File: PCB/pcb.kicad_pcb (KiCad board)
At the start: 2 copper layers, 40.2 x 62.5 mm, 7 parts, among them SW1 SW_Push, SW2 SW_Push, SW3 SW_Push, SW4 SW_Push, U1 XIAO-RP2040-DIP

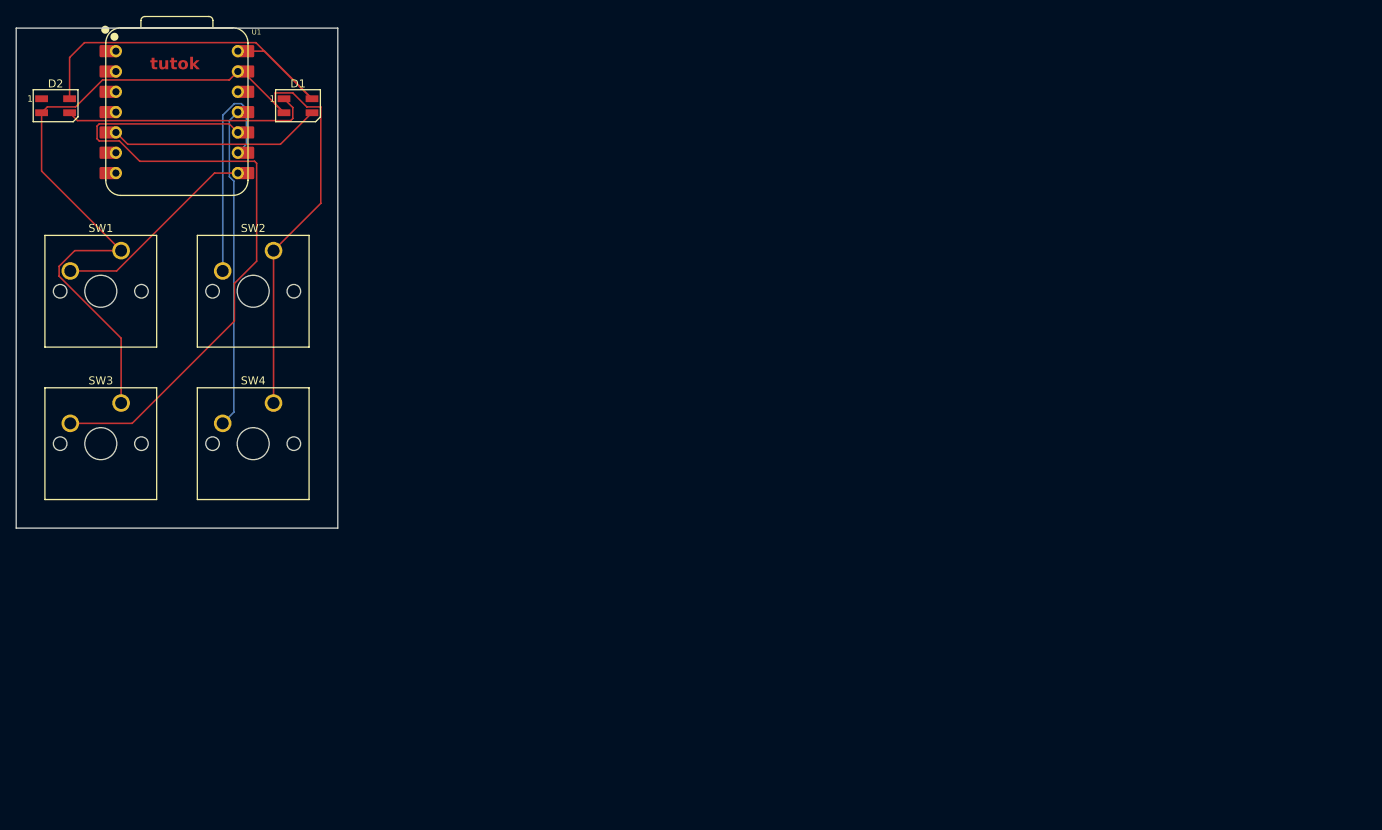
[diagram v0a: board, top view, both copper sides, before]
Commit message: Dodanie nowych plików i zmian
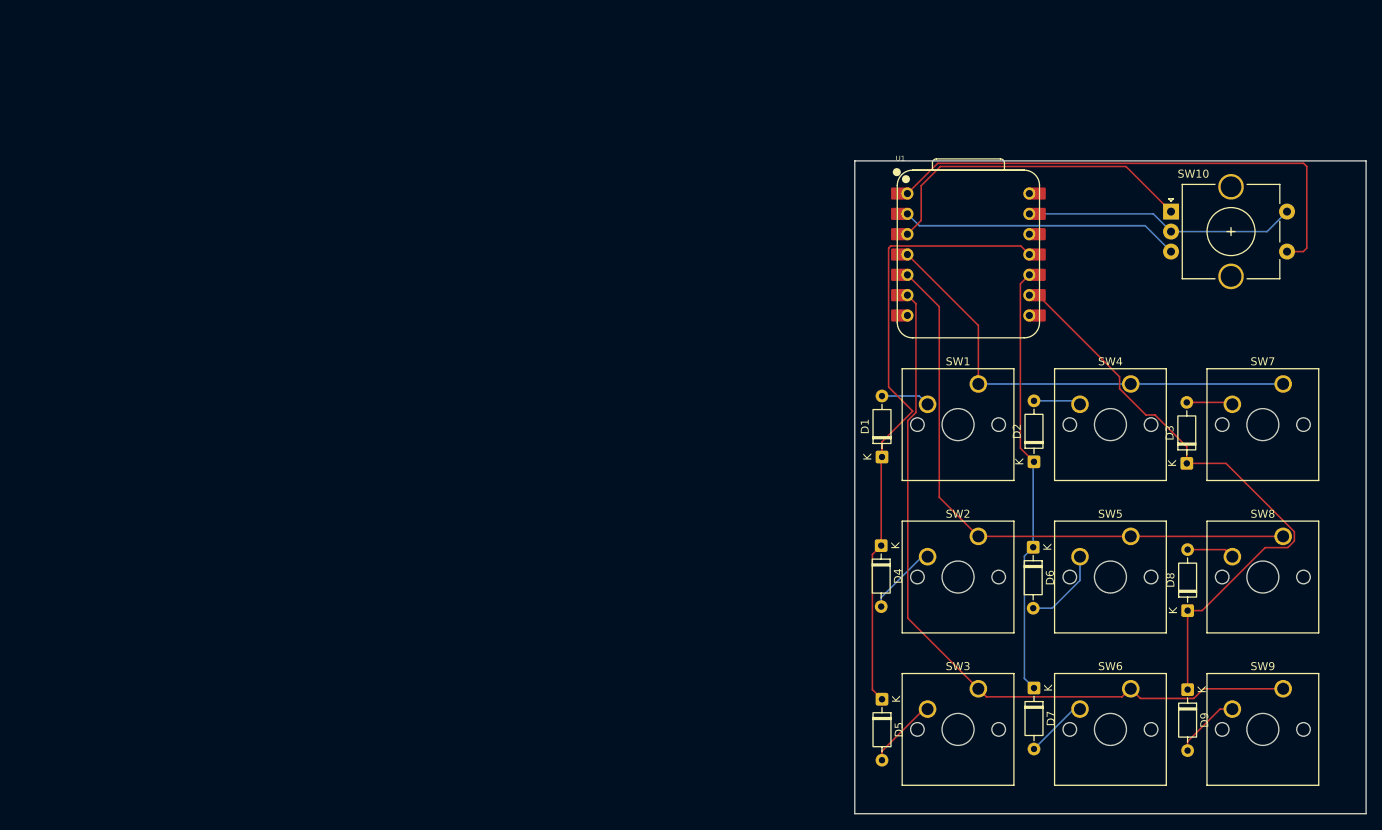
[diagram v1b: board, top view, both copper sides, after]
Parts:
- added D3: 1N4148, Diode_THT:D_DO-35_SOD27_P7.62mm_Horizontal, F.Cu at (192.9, 85.8)
- added D4: 1N4148, Diode_THT:D_DO-35_SOD27_P7.62mm_Horizontal, F.Cu at (154.7, 96.1)
- added D5: 1N4148, Diode_THT:D_DO-35_SOD27_P7.62mm_Horizontal, F.Cu at (154.8, 115.3)
- added D6: 1N4148, Diode_THT:D_DO-35_SOD27_P7.62mm_Horizontal, F.Cu at (173.7, 96.3)
- added D7: 1N4148, Diode_THT:D_DO-35_SOD27_P7.62mm_Horizontal, F.Cu at (173.8, 113.9)
- added D8: 1N4148, Diode_THT:D_DO-35_SOD27_P7.62mm_Horizontal, F.Cu at (193.0, 104.2)
- added D9: 1N4148, Diode_THT:D_DO-35_SOD27_P7.62mm_Horizontal, F.Cu at (193.0, 114.1)
- added SW10: RotaryEncoder_Switch, Rotary_Encoder:RotaryEncoder_Alps_EC11E-Switch_Vertical_H20mm_CircularMountingHoles, F.Cu at (190.9, 54.3)
- added SW5: SW_Push, Button_Switch_Keyboard:SW_Cherry_MX_1.00u_PCB, F.Cu at (185.9, 94.9)
- added SW6: SW_Push, Button_Switch_Keyboard:SW_Cherry_MX_1.00u_PCB, F.Cu at (185.9, 114.0)
- added SW7: SW_Push, Button_Switch_Keyboard:SW_Cherry_MX_1.00u_PCB, F.Cu at (204.9, 75.9)
- added SW8: SW_Push, Button_Switch_Keyboard:SW_Cherry_MX_1.00u_PCB, F.Cu at (204.9, 94.9)
- added SW9: SW_Push, Button_Switch_Keyboard:SW_Cherry_MX_1.00u_PCB, F.Cu at (204.9, 114.0)
- D1, D2: value SK6812MINI -> 1N4148; footprint LED_SMD:LED_SK6812MINI_PLCC4_3.5x3.5mm_P1.75mm -> Diode_THT:D_DO-35_SOD27_P7.62mm_Horizontal
- moved D2 130.1 mm to (173.8, 85.6), turned to 90 degrees
- moved SW3 113.0 mm to (166.8, 114.0)
- moved SW1 108.4 mm to (166.8, 75.9)
- moved SW4 107.2 mm to (185.9, 75.9)
- moved U1 100.5 mm to (165.6, 59.7)
- moved SW2 95.1 mm to (166.8, 94.9)
- moved D1 85.2 mm to (154.8, 85.0), turned to 90 degrees
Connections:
- D1 pad 1: Net-(D1-DOUT) -> ROW1
- D1 pad 2: GND -> Net-(D1-A)
- D2 pad 1: unconnected-(D2-DOUT-Pad1) -> ROW2
- D2 pad 2: GND -> Net-(D2-A)
- SW1 pad 1: GND -> COL1
- SW1 pad 2: Net-(U1-GPIO1/RX) -> Net-(D1-A)
- SW2 pad 1: GND -> COL2
- SW2 pad 2: Net-(U1-GPIO2/SCK) -> Net-(D4-A)
- SW3 pad 1: GND -> COL3
- SW3 pad 2: Net-(U1-GPIO4/MISO) -> Net-(D5-A)
- SW4 pad 1: GND -> COL1
- SW4 pad 2: Net-(U1-GPIO3/MOSI) -> Net-(D2-A)
- U1 pad 1: unconnected-(U1-GPIO26/ADC0/A0-Pad1) -> Net-(U1-GPIO26/ADC0/A0)
- U1 pad 10: Net-(U1-GPIO4/MISO) -> ROW2
- U1 pad 11: Net-(U1-GPIO3/MOSI) -> ROW1
- U1 pad 2: unconnected-(U1-GPIO27/ADC1/A1-Pad2) -> Net-(U1-GPIO27/ADC1/A1)
- U1 pad 3: unconnected-(U1-GPIO28/ADC2/A2-Pad3) -> Net-(U1-GPIO28/ADC2/A2)
- U1 pad 4: unconnected-(U1-GPIO29/ADC3/A3-Pad4) -> COL1
- U1 pad 5: Net-(D1-DIN) -> COL2
- U1 pad 6: unconnected-(U1-GPIO7/SCL-Pad6) -> COL3
- U1 pad 8: Net-(U1-GPIO1/RX) -> unconnected-(U1-GPIO1/RX-Pad8)
- U1 pad 9: Net-(U1-GPIO2/SCK) -> ROW3
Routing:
- net GND: track 133.7 -> 34.2 mm
- net COL3: track 0.00 -> 93.7 mm
- net Net-(U1-GPIO4/MISO): track 87.6 -> 0.00 mm
- net ROW1: track 0.00 -> 78.4 mm
- net ROW3: track 0.00 -> 75.5 mm
- net COL2: track 0.00 -> 74.5 mm
- net Net-(U1-GPIO26/ADC0/A0): track 0.00 -> 64.5 mm
- net COL1: track 0.00 -> 58.0 mm
- net ROW2: track 0.00 -> 53.8 mm
- net +5V: track 50.0 -> 0.00 mm
- net Net-(U1-GPIO28/ADC2/A2): track 0.00 -> 41.3 mm
- net Net-(U1-GPIO3/MOSI): track 40.2 -> 0.00 mm
- net Net-(U1-GPIO27/ADC1/A1): track 0.00 -> 34.9 mm
- net Net-(D1-DOUT): track 31.4 -> 0.00 mm
- net Net-(U1-GPIO2/SCK): track 29.2 -> 0.00 mm
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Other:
- board size 40.2 x 62.5 mm -> 63.9 x 81.6 mm
- board text removed: "tutok"
